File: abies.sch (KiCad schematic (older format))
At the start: 6 parts

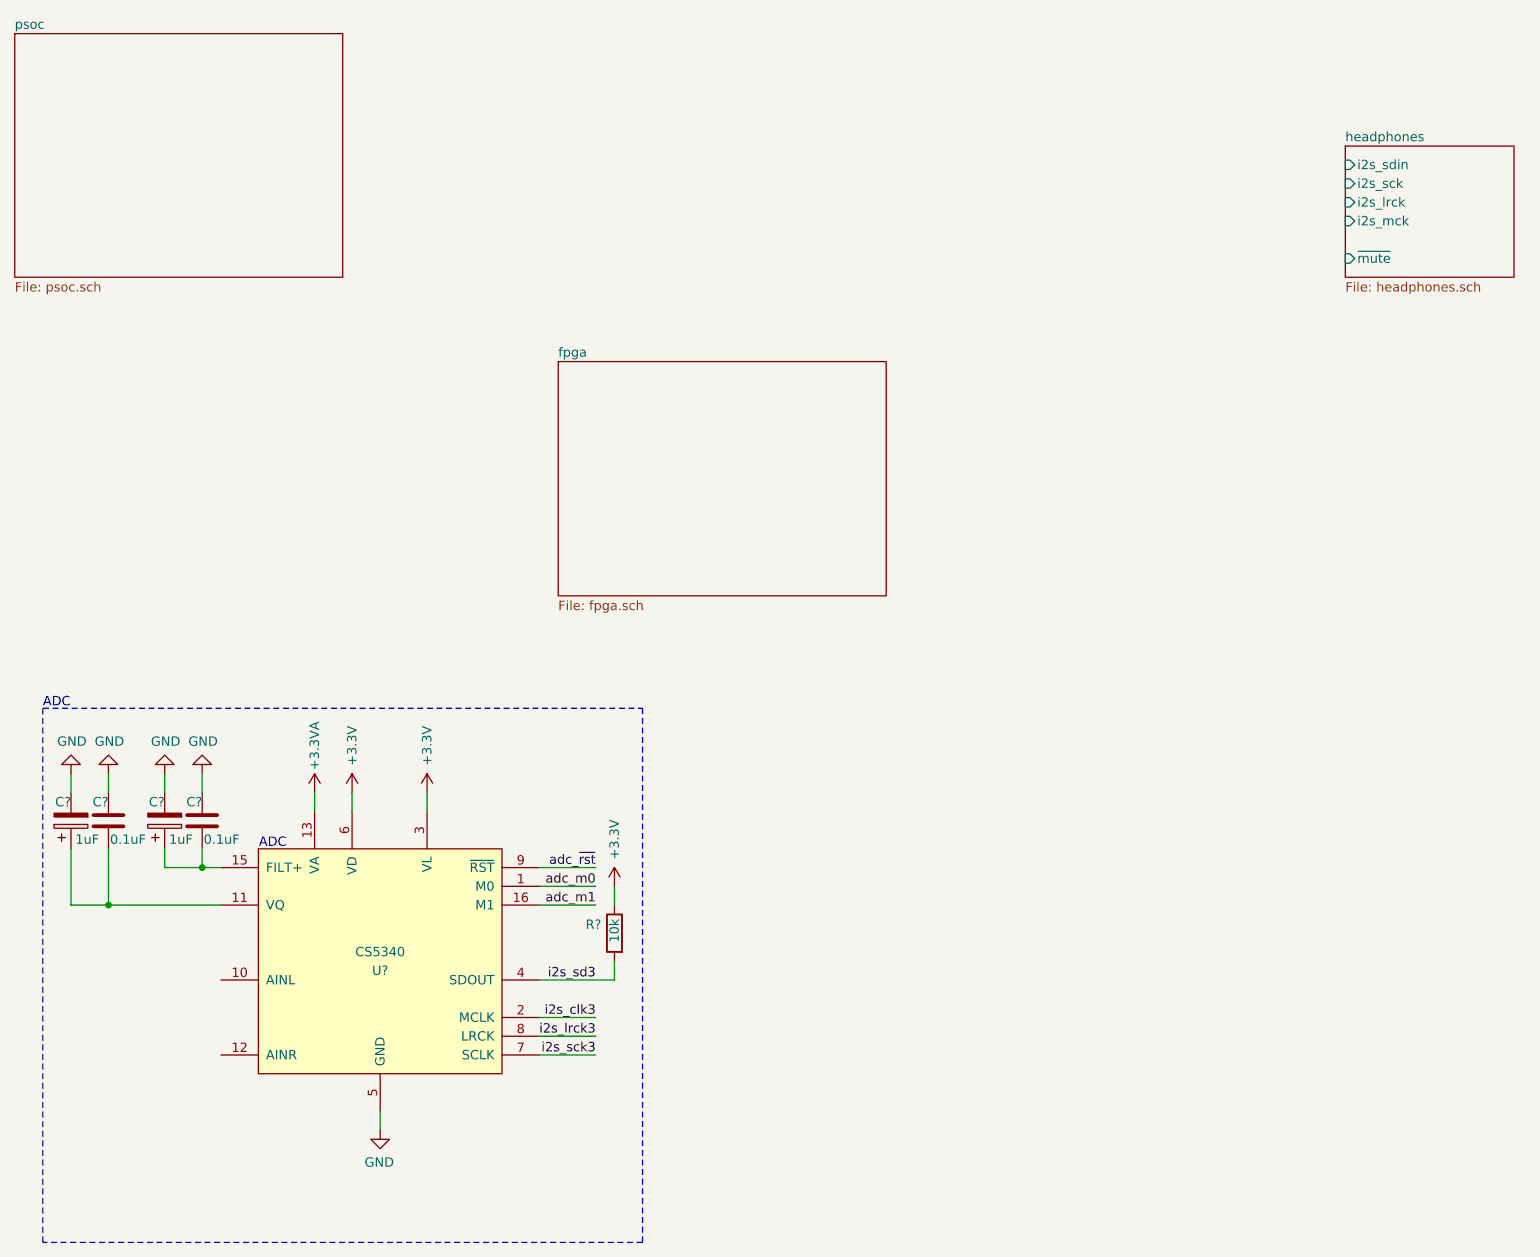
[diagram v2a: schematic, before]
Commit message: ..
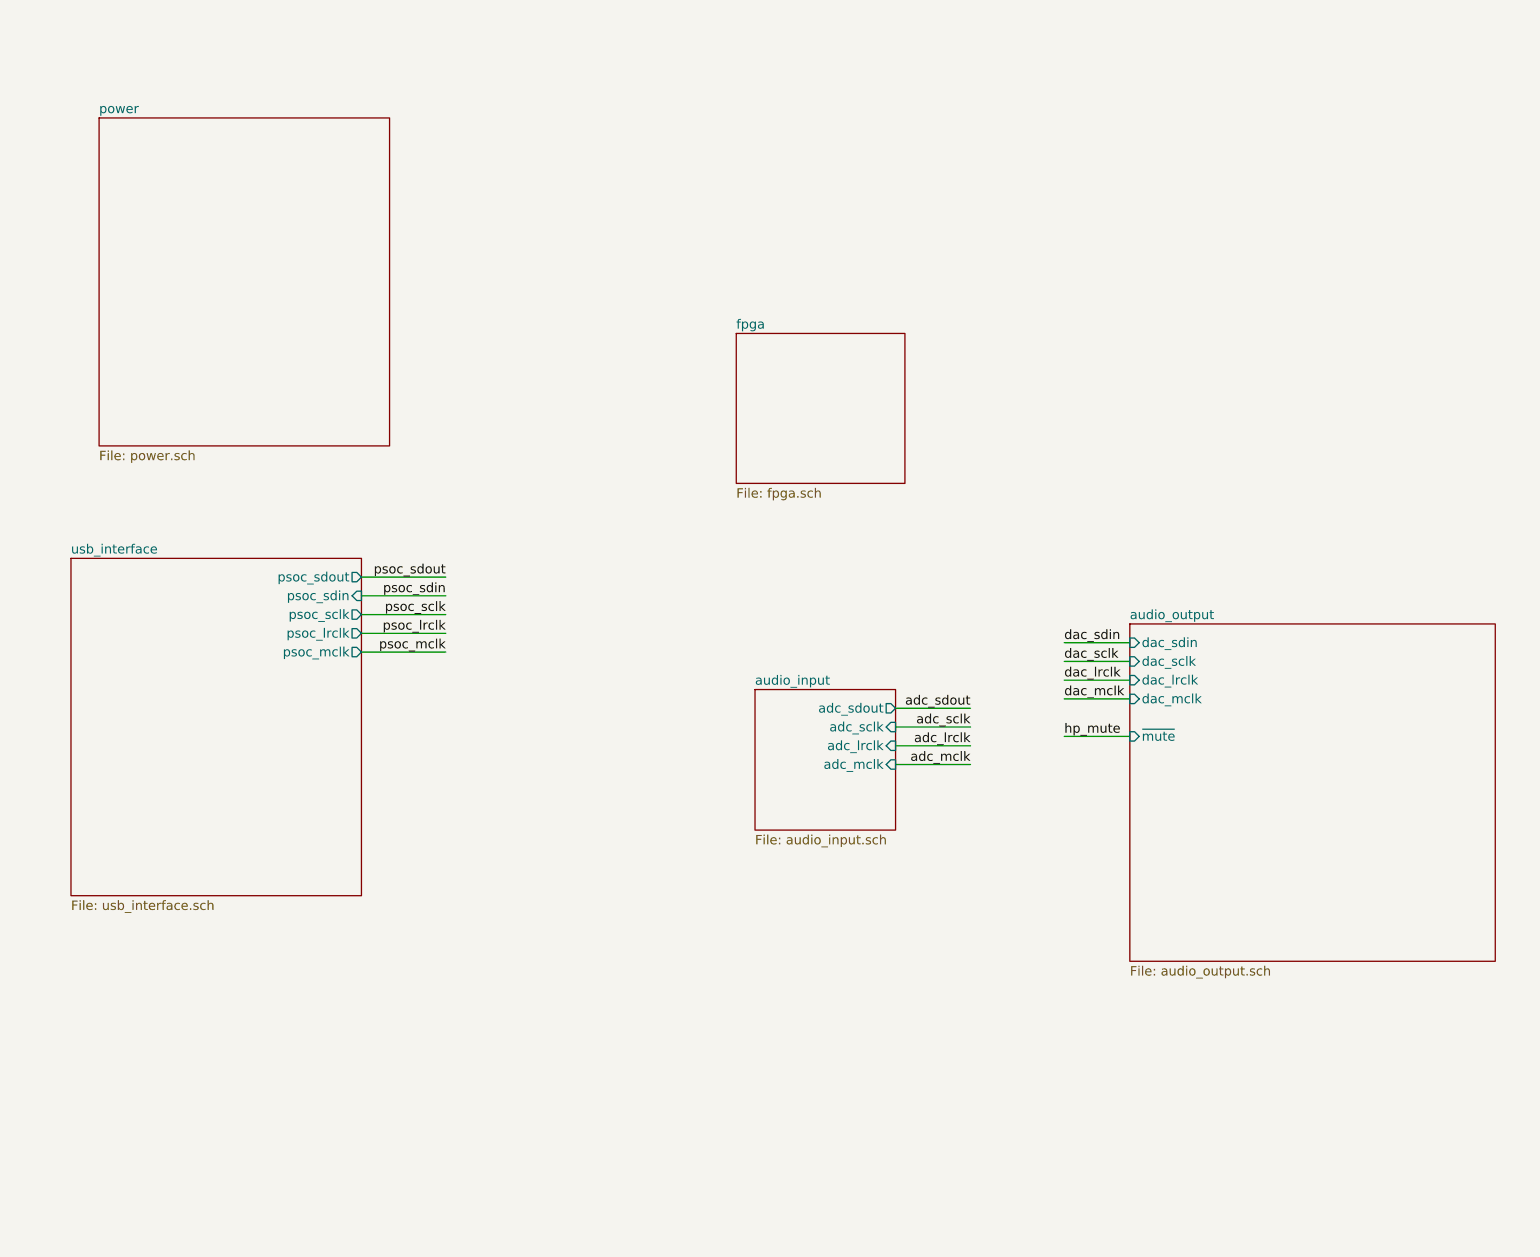
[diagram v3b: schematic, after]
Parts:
- removed C? (x2): 1uF, symbol Device:CP
- removed C? (x2): 0.1uF, symbol Device:C
- removed R?: 10k, symbol Device:R
- removed U?: CS5340, Package_SO:TSSOP-16_4.4x5mm_P0.65mm, symbol audio_digital:CS5340
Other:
- note removed: "ADC"
